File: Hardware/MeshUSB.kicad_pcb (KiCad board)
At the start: 2 copper layers, 30.2 x 44.3 mm, 42 parts, among them P1 USB_4, P2 PVCell, Q1 MOS_P, U1 XBEE, U2 AP7313-3.3VREGULATOR, U4 FT231X-SSOP, U5 LTC4070

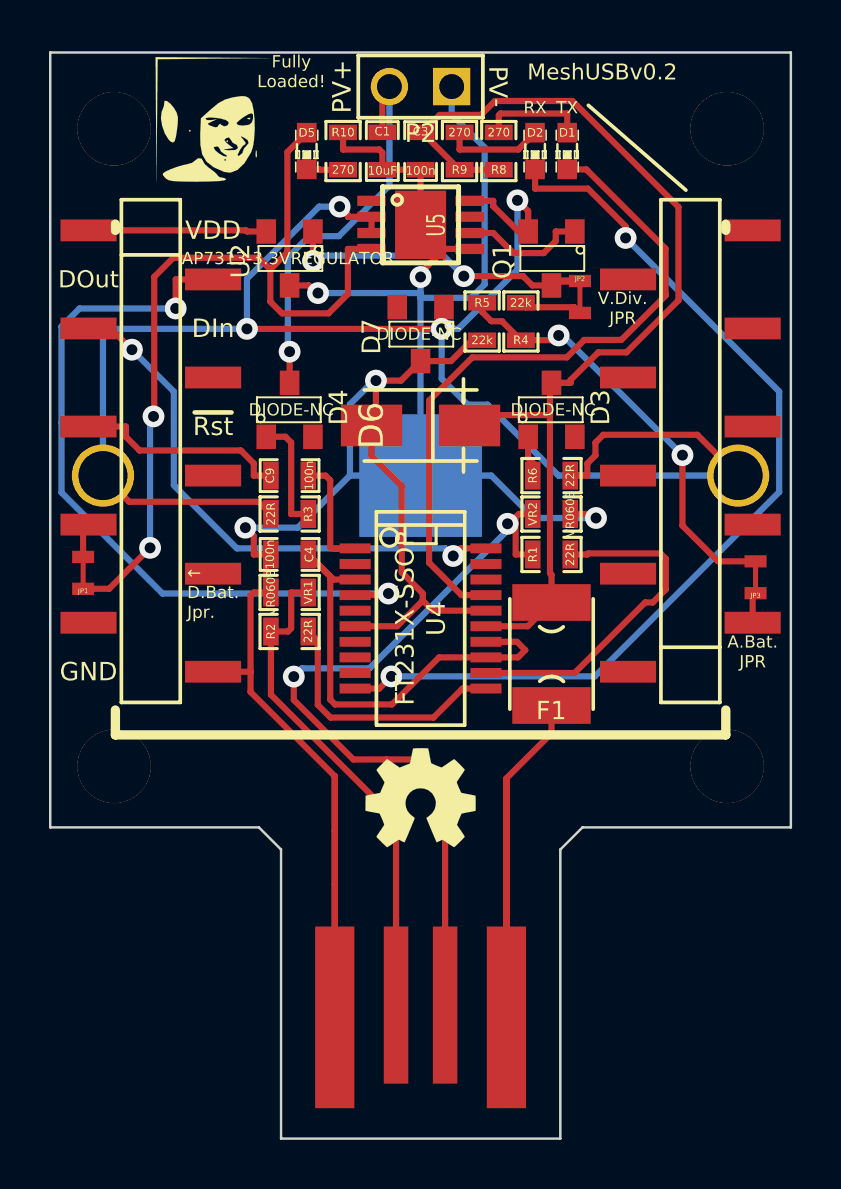
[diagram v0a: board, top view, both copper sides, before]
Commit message: Change all the things\!
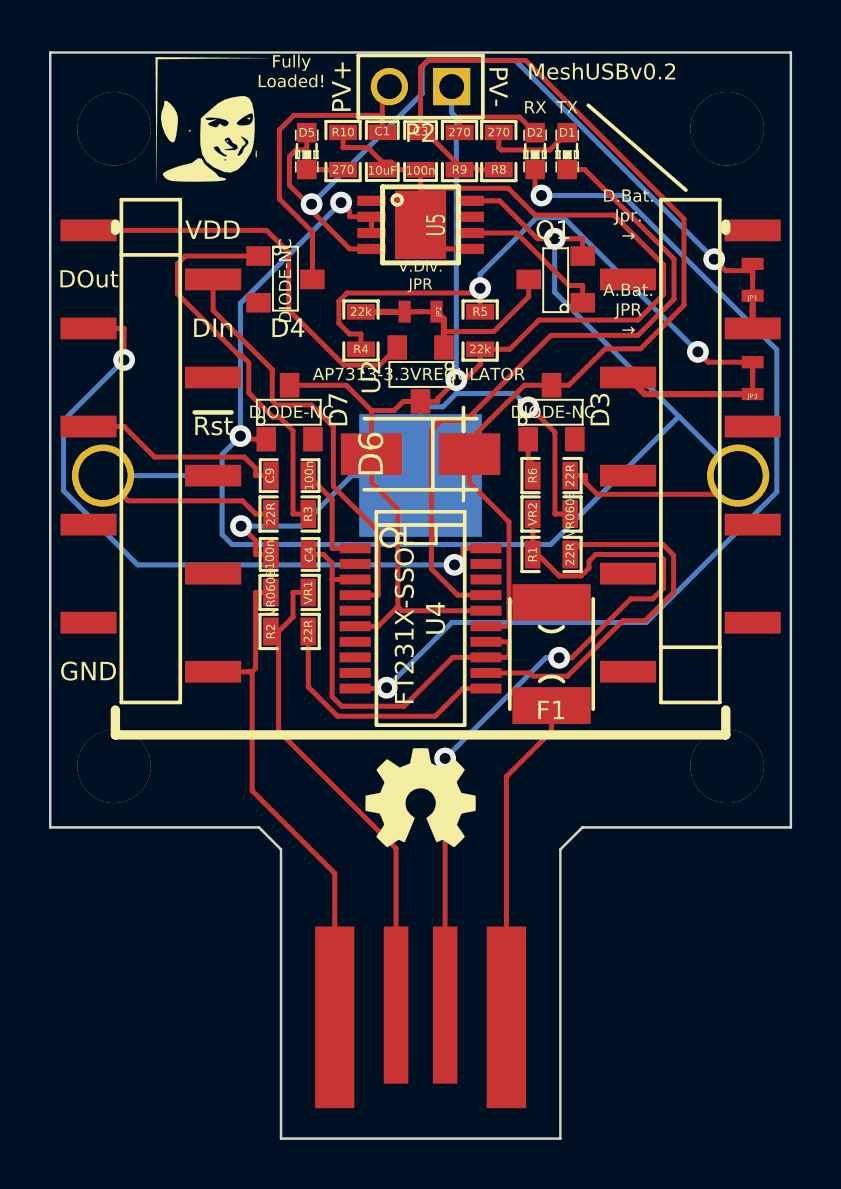
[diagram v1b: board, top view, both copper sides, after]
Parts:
- moved JP1 29.8 mm to (162.0, 107.0)
- moved JP3 8.12 mm to (162.0, 111.0)
- moved U2 7.13 mm to (148.5, 110.9)
- moved R4 6.53 mm to (146.1, 109.1)
- moved JP2 6.53 mm to (148.5, 108.3), turned to 180 degrees
- moved D7 6.22 mm to (143.2, 112.4), turned to 0 degrees
- moved D4 5.32 mm to (143.0, 107.0), turned to 270 degrees
- moved D6 1.17 mm to (148.5, 114.1)
- moved Q1 0.87 mm to (154.0, 107.0), turned to 90 degrees
- moved R5 0.38 mm to (150.9, 109.1)
- moved D3 0.10 mm to (153.8, 112.4)
- renumbered 1PIN to 1PIN1, 1PIN to 1PIN2, 1PIN to 1PIN3, 1PIN to 1PIN4
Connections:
- net _MT_PF7 renamed _MT_PF3
- D5 pad 1: _MT_PB4 -> _MT_PF2
- H1 pad 7: N-0000019 (its old number) -> N-0000022
- H2 pad 7: N-0000069 (its old number) -> N-0000023
- H2 pad 8: N-0000068 (its old number) -> N-0000020
- JP1 pad 1: _MT_PB4 -> N-0000020
- JP1 pad 2: N-0000019 (its old number) -> _MT_PF2
- JP3 pad 1: N-0000021 -> N-0000023
- U5 pad 4: _MT_PB4 -> _MT_PF2
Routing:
- net N-0000019 (its old number): track 33.1 -> 0.00 mm, vias 2 -> 0
- net _MT_PF2: track 0.00 -> 33.1 mm, vias 0 -> 2
- net N-000007: track 30.9 -> 17.4 mm, vias 2 -> 0
- net N-0000035: track 4.73 -> 16.4 mm
- net N-0000017: track 12.8 -> 1.68 mm, vias 2 -> 0
- net _MT_PF3: track 17.7 -> 27.1 mm
- net BAT+: track 7.27 -> 16.5 mm
- net N-0000061: track 19.7 -> 13.5 mm
- net N-0000010: track 22.4 -> 28.0 mm
- net N-0000032: track 73.2 -> 78.6 mm, vias 4 -> 3
- net N-0000016: track 2.58 -> 7.42 mm
- net N-0000023: track 0.00 -> 3.49 mm
- net N-0000036: track 16.5 -> 13.1 mm, vias 1 -> 0
- net GND: track 108.9 -> 112.3 mm, vias 5 -> 3
- net USB_VDD: track 42.6 -> 45.6 mm
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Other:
- net class Default: clearance 0.254 -> 0.2032; trace_width 0.254 -> 0.2032
- rule pad_to_mask_clearance: 0 -> 0.2032
- rule trace_clearance: 0.254 -> 0.2032
- rule trace_min: 0.254 -> 0.2032
- board text added: "A.Bat. JPR →"
- board text added: "D.Bat. Jpr. →"
- board text removed: "A.Bat. JPR"
- board text removed: "← D.Bat. Jpr."
